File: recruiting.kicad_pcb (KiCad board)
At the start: 2 copper layers, 1 part

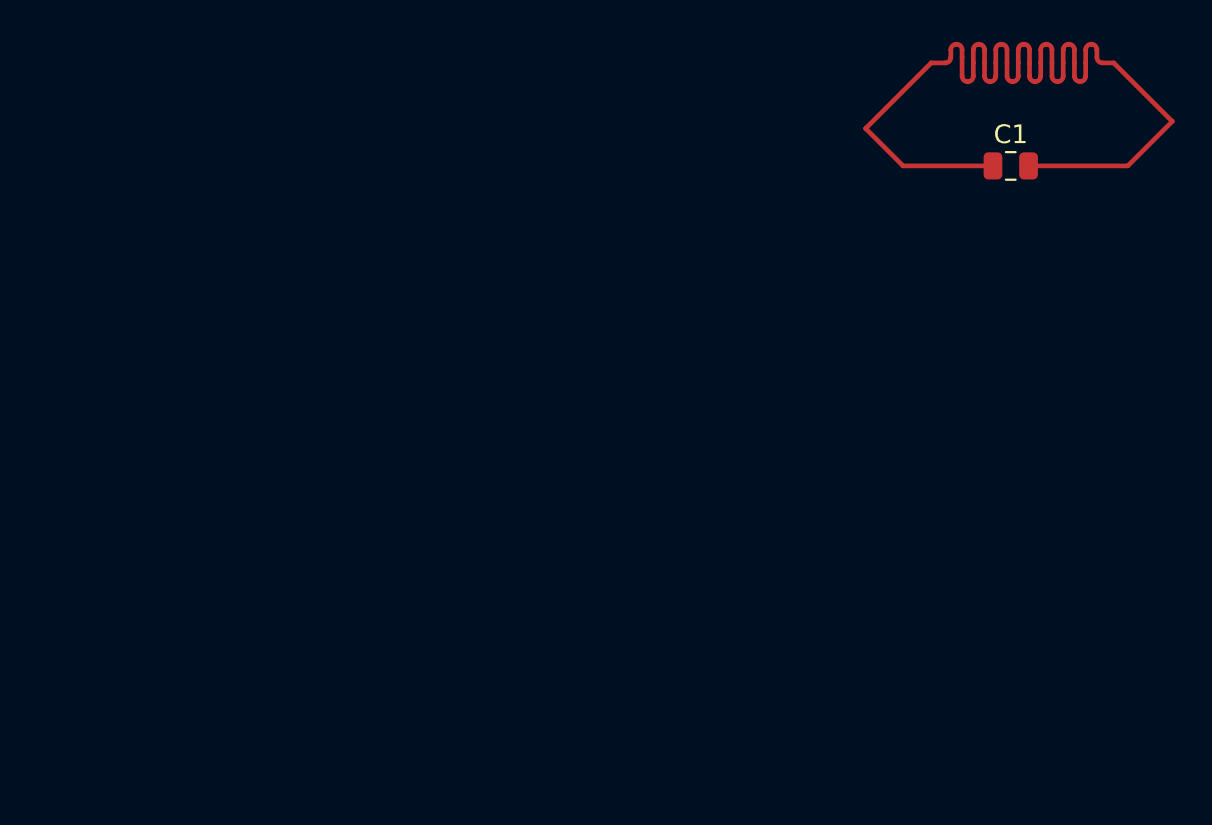
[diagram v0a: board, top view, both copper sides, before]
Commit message: Add project
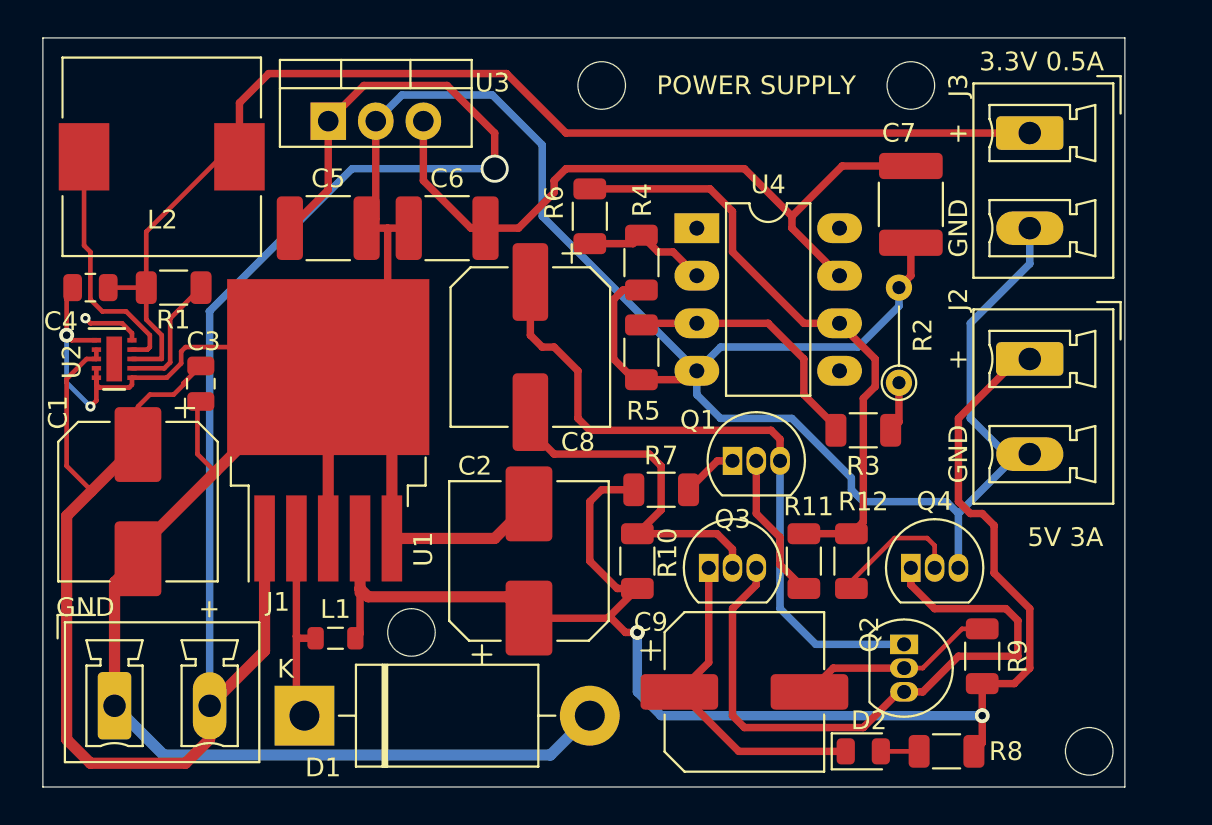
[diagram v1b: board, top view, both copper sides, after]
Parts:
- added C2: 1000uF,25V, Capacitor_SMD:CP_Elec_8x6.5, F.Cu at (125.0, 109.8)
- added C3: 2.2uF, Capacitor_SMD:C_0805_2012Metric, F.Cu at (107.5, 100.4)
- added C4: 2.2uF, Capacitor_SMD:C_0805_2012Metric, F.Cu at (101.6, 95.2)
- added C5: 0.33uF, Capacitor_SMD:C_1812_4532Metric, F.Cu at (114.3, 92.1)
- added C6: 0.1uF, Capacitor_SMD:C_1812_4532Metric, F.Cu at (120.7, 92.1)
- added C7: 0.1uF, Capacitor_SMD:C_1812_4532Metric, F.Cu at (145.4, 90.8)
- added C8: 56uF, Capacitor_SMD:CP_Elec_8x11.9, F.Cu at (125.1, 98.4)
- added C9: 56uF, Capacitor_SMD:CP_Elec_8x11.9, F.Cu at (136.5, 116.8)
- added D1: MBR340, Diode_THT:D_DO-201AD_P15.24mm_Horizontal, F.Cu at (113.0, 118.1)
- added D2: LED, LED_SMD:LED_0805_2012Metric, F.Cu at (142.9, 120.0)
- added J1: Morsetto 11-27V, Connector_Phoenix_MC_HighVoltage:PhoenixContact_MCV_1,5_2-G-5.08_1x02_P5.08mm_Vertical, F.Cu at (102.9, 117.6)
- added J2: Morsetto 5V3A, Connector_Phoenix_MC_HighVoltage:PhoenixContact_MCV_1,5_2-G-5.08_1x02_P5.08mm_Vertical, F.Cu at (151.8, 99.1)
- added J3: Morsetto 3,3V 0,5A, Connector_Phoenix_MC_HighVoltage:PhoenixContact_MCV_1,5_2-G-5.08_1x02_P5.08mm_Vertical, F.Cu at (151.8, 87.0)
- added L1: 100uH, Inductor_SMD:L_0805_2012Metric, F.Cu at (114.7, 114.0)
- added L2: 10uH, Inductor_SMD:L_10.4x10.4_H4.8, F.Cu at (105.4, 88.3)
- added Q1: BC547, Package_TO_SOT_THT:TO-92_Inline, F.Cu at (135.9, 104.5)
- added Q2: BC547, Package_TO_SOT_THT:TO-92_Inline, F.Cu at (145.1, 114.3)
- added Q3: BC547, Package_TO_SOT_THT:TO-92_Inline, F.Cu at (134.6, 110.2)
- added Q4: BC547, Package_TO_SOT_THT:TO-92_Inline, F.Cu at (145.4, 110.2)
- added R1: 100K, Resistor_SMD:R_1206_3216Metric, F.Cu at (106.0, 95.2)
- added R10: 5.6K, Resistor_SMD:R_1206_3216Metric, F.Cu at (130.8, 109.9)
- added R11: 160k, Resistor_SMD:R_1206_3216Metric, F.Cu at (139.7, 109.9)
- added R12: 56K, Resistor_SMD:R_1206_3216Metric, F.Cu at (142.2, 109.9)
- added R2: MP930-0.050-1%, Resistor_THT:R_Axial_DIN0204_L3.6mm_D1.6mm_P5.08mm_Vertical, F.Cu at (144.8, 100.3)
- added R3: 1k, Resistor_SMD:R_1206_3216Metric, F.Cu at (142.9, 102.9)
- added R4: 1k, Resistor_SMD:R_1206_3216Metric, F.Cu at (131.0, 93.9)
- added R5: 5k, Resistor_SMD:R_1206_3216Metric, F.Cu at (131.0, 98.7)
- added R6: 5k, Resistor_SMD:R_1206_3216Metric, F.Cu at (128.3, 91.4)
- added R7: 270, Resistor_SMD:R_1206_3216Metric, F.Cu at (132.1, 106.0)
- added R8: 270, Resistor_SMD:R_1206_3216Metric, F.Cu at (147.3, 120.0)
- added R9: 5.6K, Resistor_SMD:R_1206_3216Metric, F.Cu at (149.2, 114.9)
- added U1: LM2576S-5, Package_TO_SOT_SMD:TO-263-5_TabPin3, F.Cu at (114.3, 102.9)
- added U2: TPS62177DQC, Package_SON:WSON-10-1EP_2x3mm_P0.5mm_EP0.84x2.4mm, F.Cu at (102.9, 99.1)
- added U3: LM7808_TO220, Package_TO_SOT_THT:TO-220-3_Vertical, F.Cu at (114.3, 86.4)
- added U4: LM741, Package_DIP:DIP-8_W7.62mm_LongPads, F.Cu at (134.0, 92.1)
- C1: value 1F -> 100uF,75V; footprint Capacitor_SMD:C_0805_2012Metric -> Capacitor_SMD:CP_Elec_8x6.2
- moved C1 49.9 mm to (104.1, 106.7), turned to -90 degrees
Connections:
- C1 pad 1: Net-(C1-Pad1) -> /DC INPUT
- C1 pad 2: Net-(C1-Pad1) -> GND
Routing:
- net GND: track 0.00 -> 219.0 mm, vias 0 -> 2
- net /DC INPUT: track 0.00 -> 112.2 mm, vias 0 -> 1
- net /5V3A: track 0.00 -> 84.4 mm, vias 0 -> 2
- net /3.3V0.5A: track 0.00 -> 67.6 mm, vias 0 -> 1
- net Net-(C1-Pad1): track 57.5 -> 0.00 mm
- net /Alimentatore 8V1/8V: track 0.00 -> 38.3 mm
- net Net-(C8-Pad1): track 0.00 -> 36.4 mm
- net Net-(Q2-Pad3): track 0.00 -> 34.8 mm
- net /Led control/POWER METER: track 0.00 -> 32.7 mm
- net Net-(C8-Pad2): track 0.00 -> 19.3 mm
- net Net-(C9-Pad1): track 0.00 -> 17.5 mm
- net Net-(R3-Pad1): track 0.00 -> 14.0 mm
- net Net-(L2-Pad1): track 0.00 -> 13.4 mm
- net Net-(D1-Pad1): track 0.00 -> 10.7 mm
- net Net-(C9-Pad2): track 0.00 -> 10.6 mm
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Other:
- board outline added: 57.8 x 40 mm
- board text added: "+"
- board text added: "3.3V 0.5A"
- board text added: "5V 3A"
- board text added: "GND"
- board text added: "POWER SUPPLY"
